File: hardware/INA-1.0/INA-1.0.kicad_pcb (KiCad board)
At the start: 2 copper layers, 25.4 x 25.4 mm, 10 parts, among them J1 Conn_01x04, U1 AD623, U2 MCP1501-12xSN

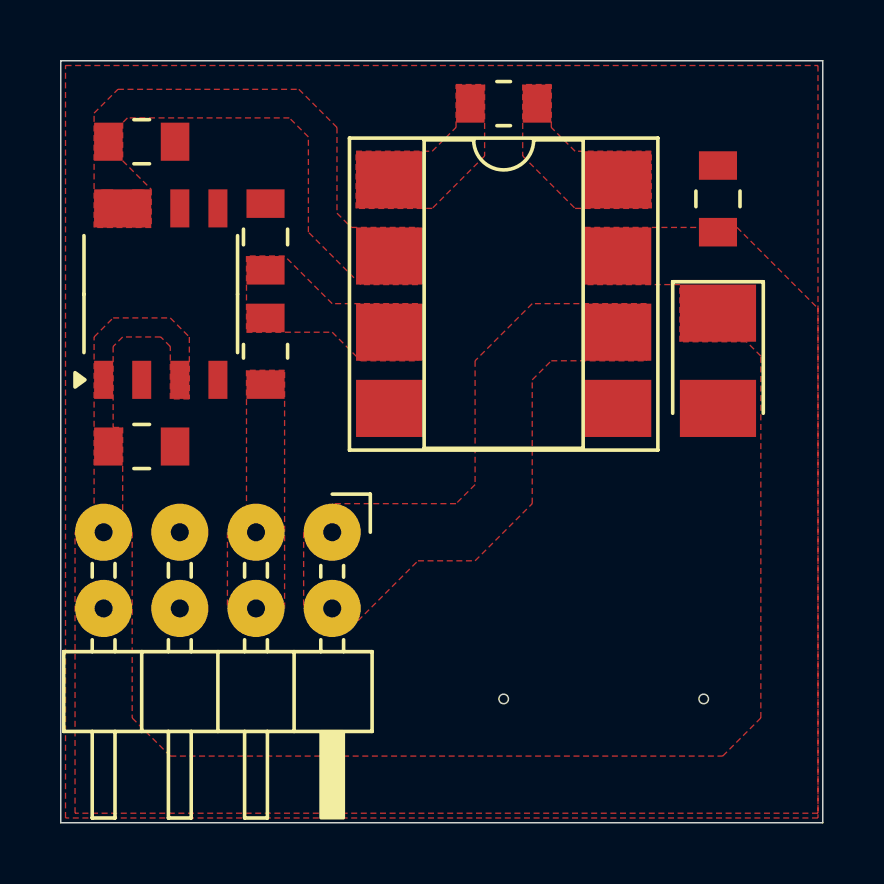
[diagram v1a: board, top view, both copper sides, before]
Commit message: new file:   hardware/CTL-5.0/CTL-5.0-backups/CTL-5.0-2026-04-14_112836.zip 	new file:   hardware/CTL-5.0/CTL-5.0-backups/CTL-5.0-2026-04-14_114223.zip 	deleted:    hardware/INA-1.0/INA-1.0-backups/INA-1.0-2026-04-13_112658.zip 	new file:   hardware/INA-1.0/INA-1.0-backups/INA-1.0-2026-04-14_092403.zip 	new file:   hardware/INA-1.0/INA-1.0-backups/INA-1.0-2026-04-14_112617.zip 	new file:   hardware/INA-1.0/INA-1.0-backups/INA-1.0-2026-04-15_103830.zip 	new file:   hardware/INA-1.0/INA-1.0-backups/INA-1.0-2026-04-15_105330.zip 	new file:   hardware/INA-1.0/INA-1.0-backups/INA-1.0-2026-04-15_110411.zip 	new file:   hardware/INA-1.0/INA-1.0-backups/INA-1.0-2026-04-15_111143.zip 	new file:   hardware/INA-1.0/INA-1.0-backups/INA-1.0-2026-04-15_111849.zip 	new file:   hardware/INA-1.0/INA-1.0-backups/INA-1.0-2026-04-15_113315.zip 	modified:   hardware/INA-1.0/INA-1.0.kicad_pcb 	modified:   hardware/INA-1.0/INA-1.0.kicad_pro 	modified:   hardware/INA-1.0/INA-1.0.kicad_sch 	new file:   hardware/INA-1.0/_autosave-INA-1.0.kicad_pcb 	modified:   hardware/INA-1.0/fabrication-outputs/INA-1.0-F_Cu.dxf 	modified:   hardware/INA-1.0/fabrication-outputs/INA-1.0-F_Mask.dxf 	new file:   hardware/INA-1.0/fabrication-outputs/TRACE-2.dwg 	new file:   hardware/INA-1.0/fabrication-outputs/TRACE-2.dxf 	new file:   hardware/INA-1.0/~INA-1.0.kicad_sch.lck 	new file:   hardware/INA-1.0/~_autosave-INA-1.0.kicad_pcb.lck 	new file:   hardware/PSU-1.0/CTL-4.3-backups/CTL-4.3-2026-01-19_105947.zip 	new file:   hardware/PSU-1.0/CTL-4.3-backups/CTL-4.3-2026-01-19_110601.zip 	new file:   hardware/PSU-1.0/CTL-4.3-backups/CTL-4.3-2026-01-19_111804.zip 	new file:   hardware/PSU-1.0/CTL-4.3-backups/CTL-4.3-2026-01-19_113721.zip 	new file:   hardware/PSU-1.0/CTL-4.3-backups/CTL-4.3-2026-01-19_164107.zip 	new file:   hardware/PSU-1.0/CTL-4.3-backups/CTL-4.3-2026-01-20_112913.zip 	new file:   hardware/PSU-1.0/CTL-4.3-backups/CTL-4.3-2026-02-11_163805.zip 	new file:   hardware/PSU-1.0/CTL-4.3-backups/CTL-4.3-2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
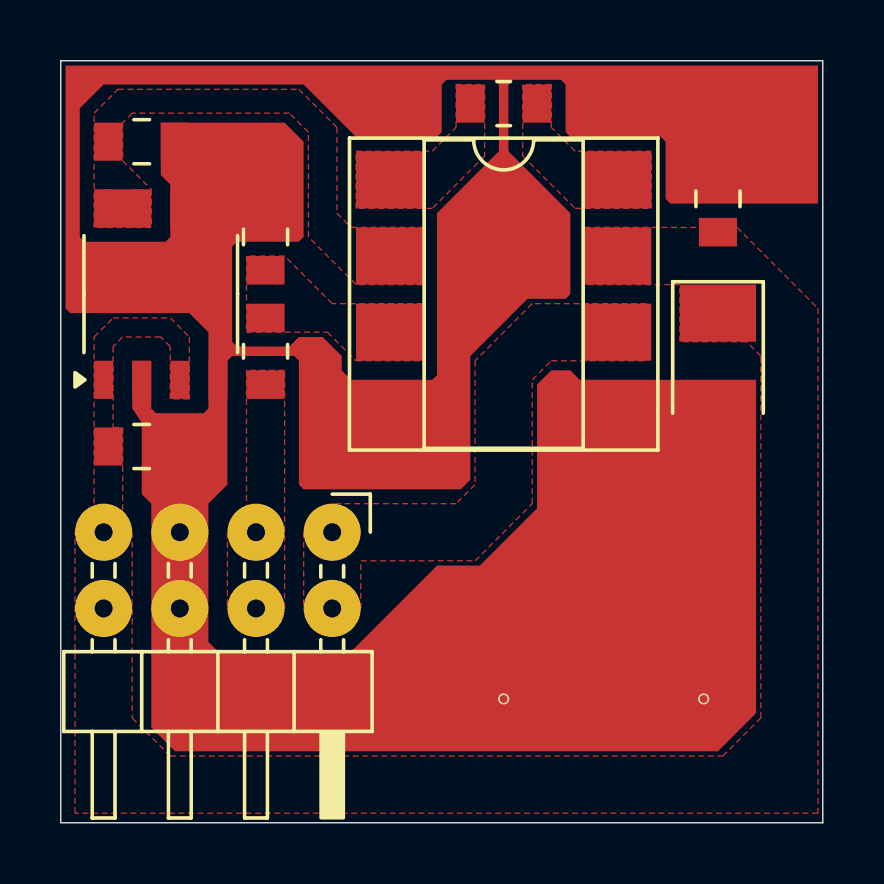
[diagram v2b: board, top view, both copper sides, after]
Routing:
- removed copper zone on F.Cu, net GND
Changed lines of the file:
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@@
 		)
 		(property "Value" "100nF"
-			(at 0 1.679999 360)
+			(at 0 1.679999 0)
 			(layer "F.Fab")
 			(effects
@@
 		)
 		(fp_text user "${REFERENCE}"
-			(at 0 0 360)
+			(at 0 0 0)
 			(layer "F.Fab")
 			(effects
@@
 		)
 		(property "Value" "2.2µF"
-			(at 0 1.679999 360)
+			(at 0 1.679999 0)
 			(layer "F.Fab")
 			(effects
@@
 		)
 		(fp_text user "${REFERENCE}"
-			(at 0 0 360)
+			(at 0 0 0)
 			(layer "F.Fab")
 			(effects
@@
 		)
 		(fp_text user "${REFERENCE}"
-			(at 5.31 3.81 360)
+			(at 5.31 3.81 0)
 			(layer "F.Fab")
 			(effects
@@
 		)
 	)
+	(gr_poly
+		(pts
+			(xy 51.27625 61.9125) (xy 51.435 62.07125) (xy 52.705 62.07125) (xy 55.40375 62.07125) (xy 56.03875 62.70625)
+			(xy 56.03875 65.24625) (xy 55.88 65.405) (xy 54.2925 65.405) (xy 54.13375 65.24625) (xy 54.13375 63.65875)
+			(xy 53.49875 63.65875) (xy 53.49875 65.24625) (xy 53.81625 65.7225) (xy 53.81625 68.10375) (xy 54.13375 68.42125)
+			(xy 54.13375 75.8825) (xy 54.9275 76.67625) (xy 73.025 76.67625) (xy 74.295 75.40625) (xy 74.295 73.3425)
+			(xy 74.295 64.29375) (xy 68.42125 64.29375) (xy 68.10375 63.97625) (xy 67.46875 63.97625) (xy 66.9925 64.4525)
+			(xy 66.9925 68.58) (xy 65.0875 70.485) (xy 63.65875 70.485) (xy 60.80125 73.3425) (xy 56.35625 73.3425)
+			(xy 56.03875 73.025) (xy 56.03875 68.42125) (xy 56.67375 67.78625) (xy 56.67375 63.65875) (xy 56.8325 63.5)
+			(xy 58.89625 63.5) (xy 59.055 63.65875) (xy 59.055 67.78625) (xy 59.21375 67.945) (xy 64.4525 67.945)
+			(xy 64.77 67.6275) (xy 64.77 63.5) (xy 66.675 61.595) (xy 67.945 61.595) (xy 68.10375 61.43625) (xy 68.10375 58.7375)
+			(xy 66.04 56.67375) (xy 65.7225 56.67375) (xy 63.65875 58.7375) (xy 63.65875 64.135) (xy 63.5 64.29375)
+			(xy 60.80125 64.29375) (xy 60.48375 63.97625) (xy 60.48375 63.5) (xy 59.84875 62.865) (xy 59.055 62.865)
+			(xy 58.7375 63.1825) (xy 56.99125 63.1825) (xy 56.8325 63.02375) (xy 56.8325 59.84875) (xy 56.99125 59.69)
+			(xy 59.055 59.69) (xy 59.21375 59.53125) (xy 59.21375 56.35625) (xy 58.57875 55.72125) (xy 54.45125 55.72125)
+			(xy 54.45125 57.4675) (xy 54.76875 57.785) (xy 54.76875 59.53125) (xy 54.61 59.69) (xy 51.91125 59.69)
+			(xy 51.7525 59.53125) (xy 51.7525 55.245) (xy 52.54625 54.45125) (xy 59.21375 54.45125) (xy 60.96 56.1975)
+			(xy 63.65875 56.1975) (xy 63.8175 56.03875) (xy 63.8175 54.45125) (xy 63.97625 54.2925) (xy 65.56375 54.2925)
+			(xy 65.7225 54.45125) (xy 65.7225 56.8325) (xy 66.04 56.8325) (xy 66.04 54.45125) (xy 66.19875 54.2925)
+			(xy 67.78625 54.2925) (xy 67.945 54.45125) (xy 67.945 56.03875) (xy 68.10375 56.1975) (xy 71.12 56.1975)
+			(xy 71.27875 56.35625) (xy 71.27875 58.26125) (xy 71.4375 58.42) (xy 76.35875 58.42) (xy 76.35875 53.81625)
+			(xy 51.27625 53.81625)
+		)
+		(stroke
+			(width 0)
+			(type solid)
+		)
+		(fill solid)
+		(layer "F.Cu")
+		(net 1)
+	)
 	(gr_rect
 		(start 59.21375 69.37375)
@@
 			(clearance 0.15875)
 		)
-		(min_thickness 0.3175)
+		(min_thickness 0.03175)
 		(filled_areas_thickness no)
 		(fill yes
@@
 			(clearance 0)
 		)
-		(min_thickness 0.3175)
+		(min_thickness 0.03175)
 		(filled_areas_thickness no)
 		(fill yes
@@
 			(pts
 				(xy 70.64375 61.75375) (xy 66.83375 61.75375) (xy 64.92875 63.65875) (xy 64.92875 67.78625) (xy 64.29375 68.42125)
-				(xy 60.16625 68.42125) (xy 60.16625 69.37375) (xy 59.21375 69.37375) (xy 59.21375 71.91375) (xy 60.16625 71.91375)
-				(xy 60.80125 72.54875) (xy 63.02375 70.32625) (xy 64.92875 70.32625) (xy 66.83375 68.42125) (xy 66.83375 64.29375)
-				(xy 67.46875 63.65875) (xy 70.64375 63.65875)
+				(xy 60.16625 68.42125) (xy 60.16625 69.37375) (xy 59.21375 69.37375) (xy 59.21375 71.91375) (xy 61.11875 71.91375)
+				(xy 61.11875 70.32625) (xy 64.92875 70.32625) (xy 66.83375 68.42125) (xy 66.83375 64.29375) (xy 67.46875 63.65875)
+				(xy 70.64375 63.65875)
 			)
 		)
@@
 	)
 	(zone
-		(net 0)
-		(net_name "")
-		(layer "F.Cu")
-		(hatch none 0.15875)
-		(connect_pads yes
-			(clearance 0)
-		)
-		(min_thickness 0.3175)
-		(filled_areas_thickness no)
-		(keepout
-			(tracks allowed)
-			(vias allowed)
-			(pads allowed)
-			(copperpour not_allowed)
-			(footprints allowed)
-		)
-		(fill
-			(thermal_gap 0.5)
-			(thermal_bridge_width 0.5)
-		)
-		(polygon
-			(pts
-				(xy 68.10375 58.57875) (xy 70.96125 58.57875) (xy 70.96125 59.21375) (xy 68.58 59.21375) (xy 68.58 61.11875)
-				(xy 71.755 61.11875) (xy 71.755 63.02375) (xy 73.9775 63.02375) (xy 74.45375 63.5) (xy 74.45375 64.29375)
-				(xy 68.42125 64.29375) (xy 68.10375 63.97625) (xy 67.31 63.97625) (xy 67.6275 63.65875) (xy 70.8025 63.65875)
-				(xy 70.8025 61.75375) (xy 68.10375 61.75375)
-			)
-		)
-	)
-	(zone
-		(net 0)
-		(net_name "")
-		(layer "F.Cu")
-		(hatch none 0.15875)
-		(connect_pads yes
-			(clearance 0)
-		)
-		(min_thickness 0.3175)
-		(filled_areas_thickness no)
-		(keepout
-			(tracks allowed)
-			(vias allowed)
-			(pads allowed)
-			(copperpour not_allowed)
-			(footprints allowed)
-		)
-		(fill
-			(thermal_gap 0.5)
-			(thermal_bridge_width 0.5)
-		)
-		(polygon
-			(pts
-				(xy 63.65875 63.97625) (xy 63.34125 64.29375) (xy 60.80125 64.29375) (xy 60.48375 63.97625) (xy 60.48375 63.1825)
-				(xy 60.96 63.65875) (xy 63.1825 63.65875) (xy 63.1825 61.75375) (xy 60.80125 61.75375) (xy 60.80125 61.11875)
-				(xy 63.1825 61.11875) (xy 63.1825 59.21375) (xy 60.96 59.21375) (xy 60.48375 58.7375) (xy 60.48375 56.515)
-				(xy 60.96 56.515) (xy 60.80125 56.67375) (xy 60.80125 58.57875) (xy 63.65875 58.57875)
-			)
-		)
-	)
-	(zone
 		(net 5)
 		(net_name "/INPUT")
@@
 			(clearance 0.15875)
 		)
-		(min_thickness 0.3175)
+		(min_thickness 0.03175)
 		(filled_areas_thickness no)
 		(fill yes
@@
 		(priority 1)
 		(connect_pads yes
-			(clearance 0.15875)
-		)
-		(min_thickness 0.3175)
+			(clearance 0)
+		)
+		(min_thickness 0.03175)
 		(filled_areas_thickness no)
 		(fill yes
@@
 			(pts
 				(xy 54.13375 59.21375) (xy 52.22875 59.21375) (xy 52.22875 55.40375) (xy 53.0225 54.61) (xy 59.055 54.61)
-				(xy 60.325 55.88) (xy 60.325 58.7375) (xy 60.80125 59.21375) (xy 63.02375 59.21375) (xy 63.02375 61.11875)
-				(xy 61.11875 61.11875) (xy 59.3725 59.3725) (xy 59.3725 56.1975) (xy 58.7375 55.5625) (xy 53.34 55.5625)
+				(xy 60.325 55.88) (xy 60.325 58.7375) (xy 60.80125 59.21375) (xy 63.1825 59.21375) (xy 63.1825 61.11875)
+				(xy 60.96 61.11875) (xy 59.3725 59.53125) (xy 59.3725 56.03875) (xy 58.7375 55.40375) (xy 53.49875 55.40375)
 				(xy 53.18125 55.72125) (xy 53.18125 56.99125) (xy 54.13375 57.94375)
 			)
@@
 			(clearance 0.15875)
 		)
-		(min_thickness 0.3175)
+		(min_thickness 0.03175)
 		(filled_areas_thickness no)
 		(fill yes
@@
 			(clearance 0.15875)
 		)
-		(min_thickness 0.3175)
+		(min_thickness 0.03175)
 		(filled_areas_thickness no)
 		(fill yes
@@
 		(polygon
 			(pts
-				(xy 63.02375 63.65875) (xy 63.02375 61.75375) (xy 60.16625 61.75375) (xy 58.57875 60.16625) (xy 57.30875 60.16625)
-				(xy 57.30875 62.70625) (xy 60.16625 62.70625) (xy 61.11875 63.65875)
-			)
-		)
-	)
-	(zone
-		(net 1)
-		(net_name "GND")
-		(layer "F.Cu")
-		(hatch none 0.15875)
-		(connect_pads yes
-			(clearance 0.15875)
-		)
-		(min_thickness 0.03175)
-		(filled_areas_thickness no)
-		(fill yes
-			(thermal_gap 0)
-			(thermal_bridge_width 0.5)
-		)
-		(polygon
-			(pts
-				(xy 51.27625 53.81625) (xy 76.35875 53.81625) (xy 76.35875 78.89875) (xy 51.27625 78.89875)
+				(xy 63.1825 63.65875) (xy 63.1825 61.75375) (xy 60.16625 61.75375) (xy 58.57875 60.16625) (xy 57.30875 60.16625)
+				(xy 57.30875 62.70625) (xy 60.0075 62.70625) (xy 60.96 63.65875)
 			)
 		)
@@
 		(priority 1)
 		(connect_pads yes
-			(clearance 0.15875)
-		)
-		(min_thickness 0.3175)
+			(clearance 0)
+		)
+		(min_thickness 0.03175)
 		(filled_areas_thickness no)
 		(fill yes
 			(thermal_gap 0.5)
 			(thermal_bridge_width 0.5)
+			(smoothing chamfer)
 		)
 		(polygon
